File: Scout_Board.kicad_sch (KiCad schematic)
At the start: 3 parts, among them U1 ESP32-S3-DEVKITC-1U-N8R2

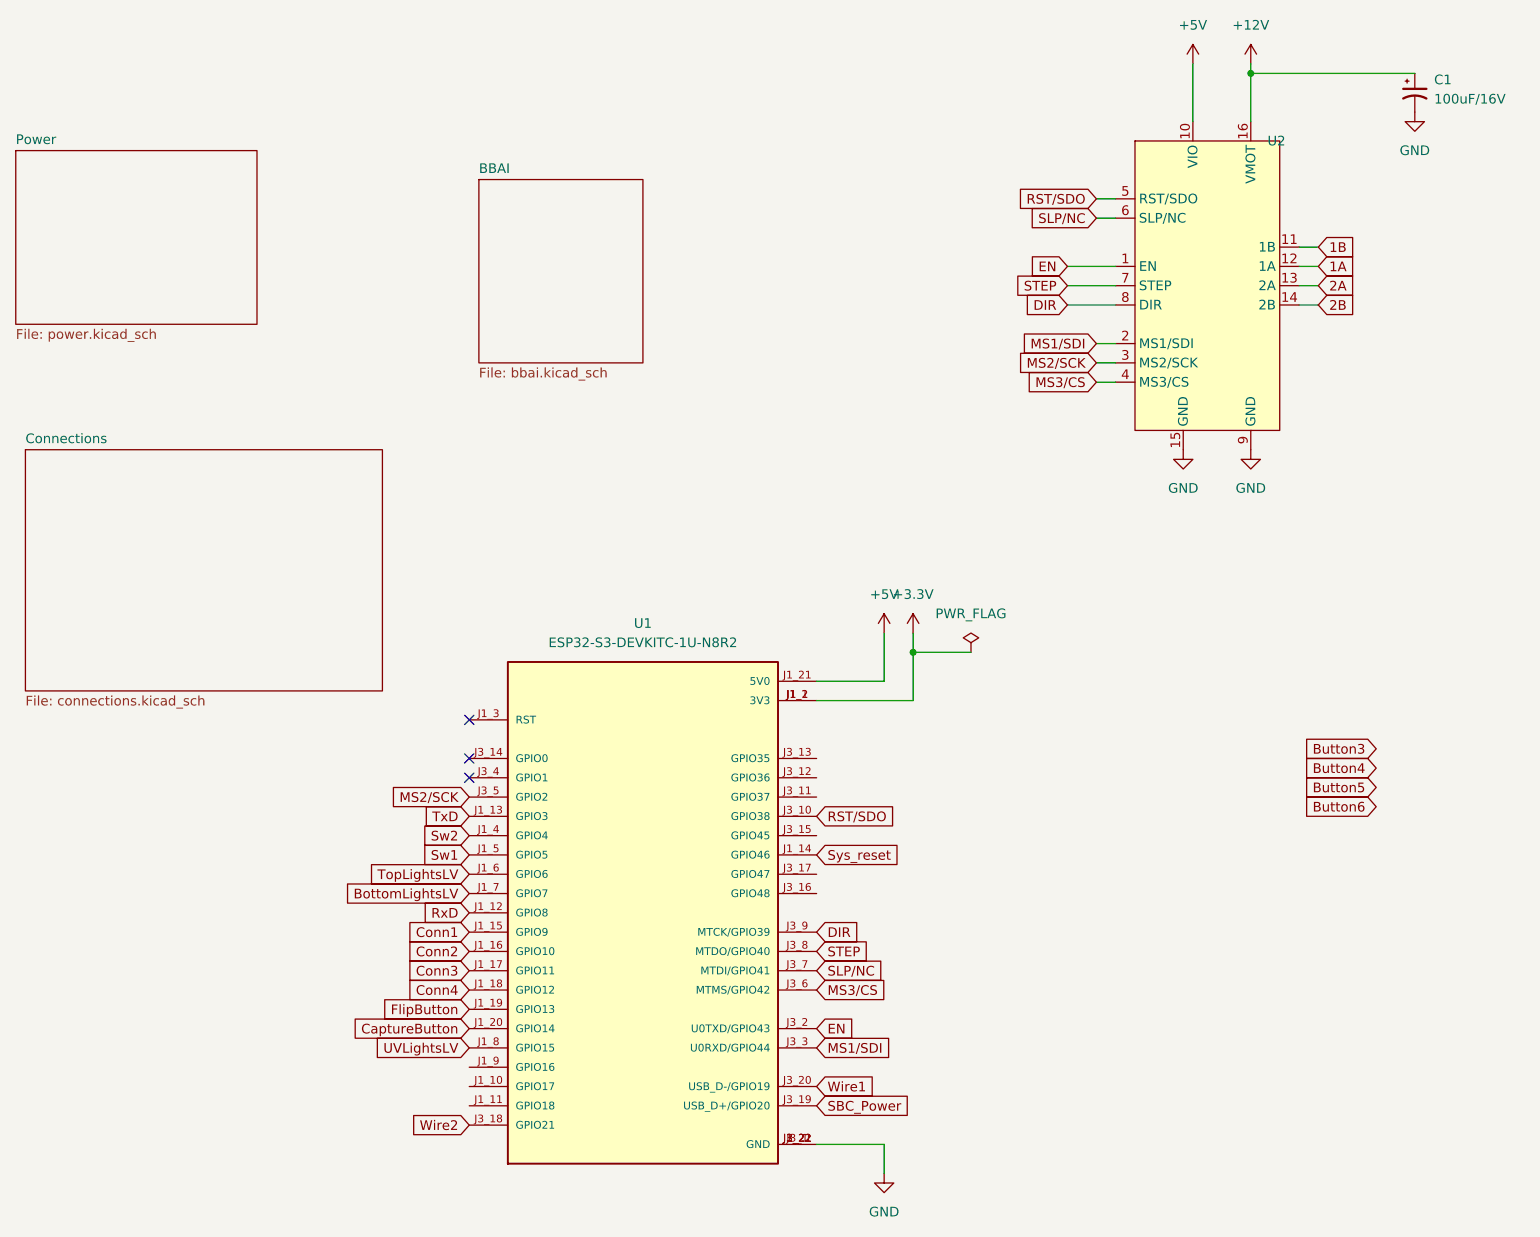
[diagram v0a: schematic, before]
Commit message: Updated board
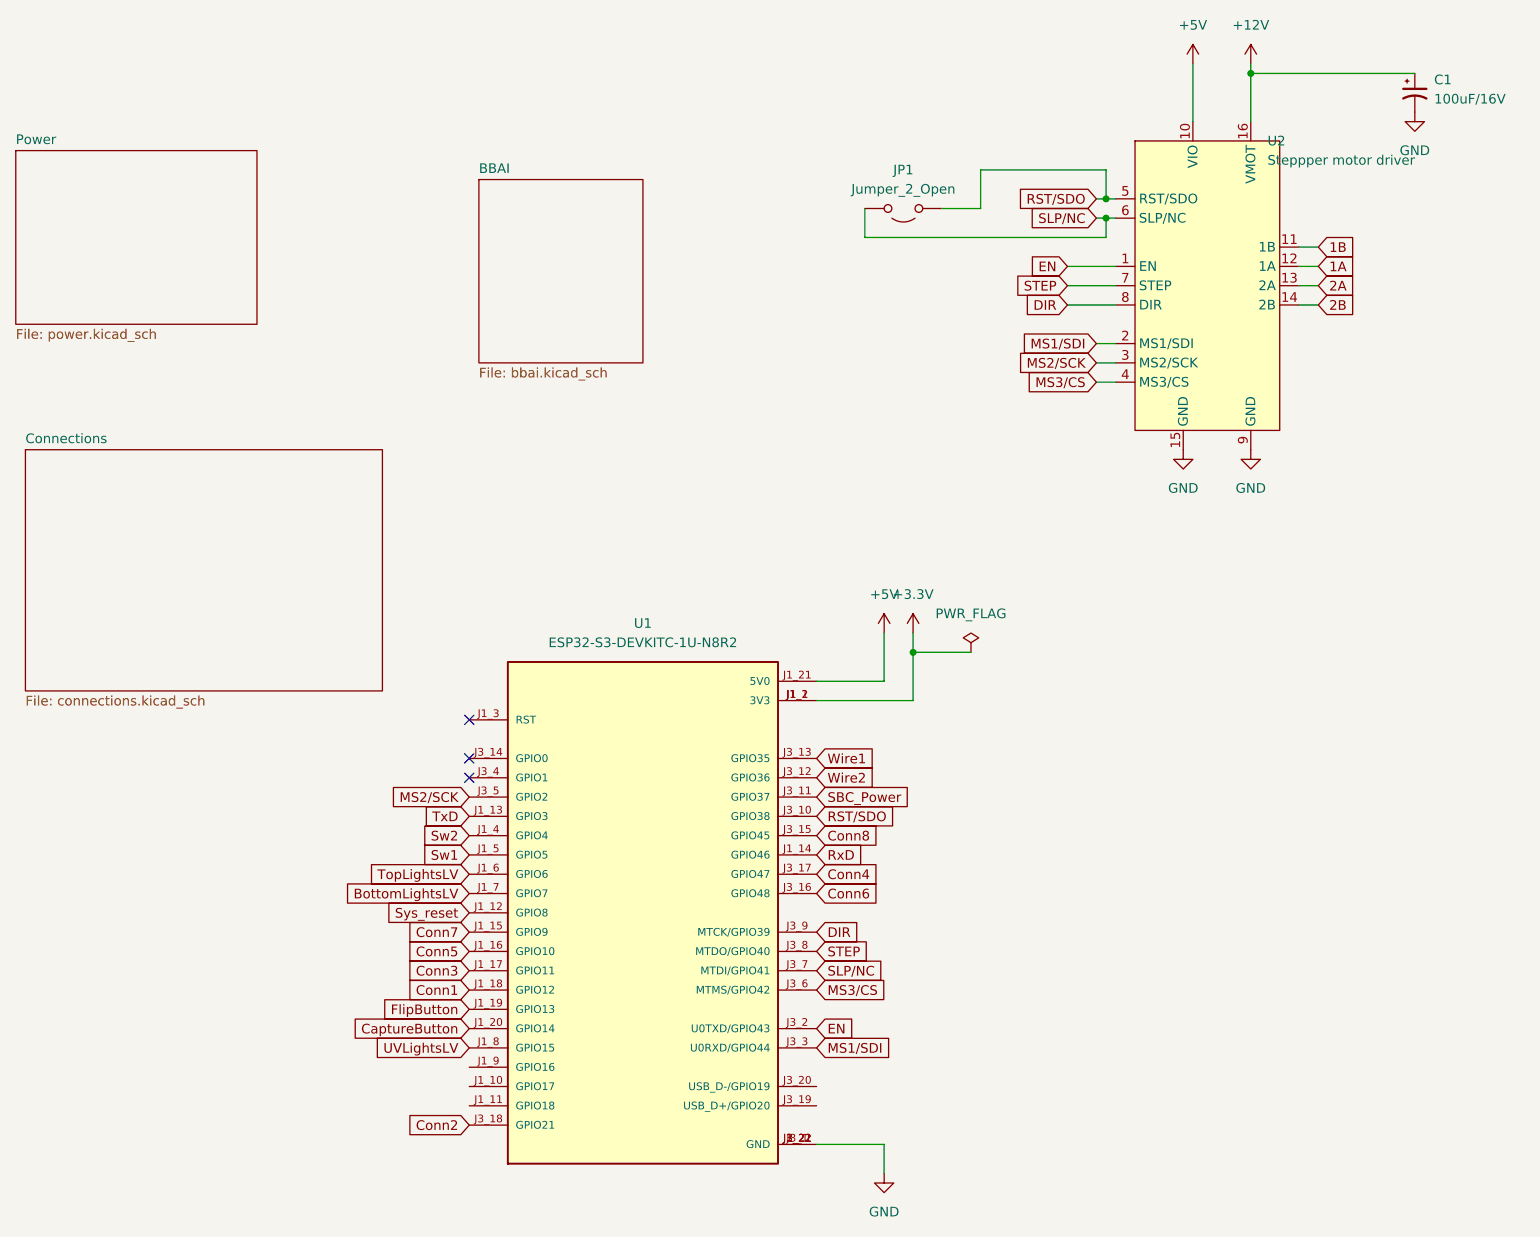
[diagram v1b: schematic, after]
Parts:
- added JP1: Jumper_2_Open, TestPoint:TestPoint_2Pads_Pitch2.54mm_Drill0.8mm, symbol Jumper:Jumper_2_Open
- C1: LCSC (none) -> C111600; Part Number (none) -> 865080343009
- U2: value ~ -> Steppper motor driver
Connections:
- net Conn1: now also U1.J1_18 (GPIO12); no longer U1.J1_15 (GPIO9)
- net Conn2: now also U1.J3_18 (GPIO21); no longer U1.J1_16 (GPIO10)
- net Conn4: now also U1.J3_17 (GPIO47); no longer U1.J1_18 (GPIO12)
- net RST/SDO: now also JP1.1 (A)
- net RxD: now also U1.J1_14 (GPIO46); no longer U1.J1_12 (GPIO8)
- net SBC_Power: now also U1.J3_11 (GPIO37); no longer U1.J3_19 (USB_D+/GPIO20)
- net SLP/NC: now also JP1.2 (B)
- net Sys_reset: now also U1.J1_12 (GPIO8); no longer U1.J1_14 (GPIO46)
- net Wire1: now also U1.J3_13 (GPIO35); no longer U1.J3_20 (USB_D-/GPIO19)
- net Wire2: now also U1.J3_12 (GPIO36); no longer U1.J3_18 (GPIO21)
- net Conn8: now reaches U1.J3_15 (GPIO45)
- net Conn6: now reaches U1.J3_16 (GPIO48)
- new net Conn5: U1.J1_16 (GPIO10)
- new net Conn7: U1.J1_15 (GPIO9)
